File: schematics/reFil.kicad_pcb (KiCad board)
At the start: 2 copper layers, 19 parts, among them CON1 BARREL_JACK, P1 CONN_5X2, P2 CONN_2, P3 CONN_2, P4 CONN_2, U1 7805

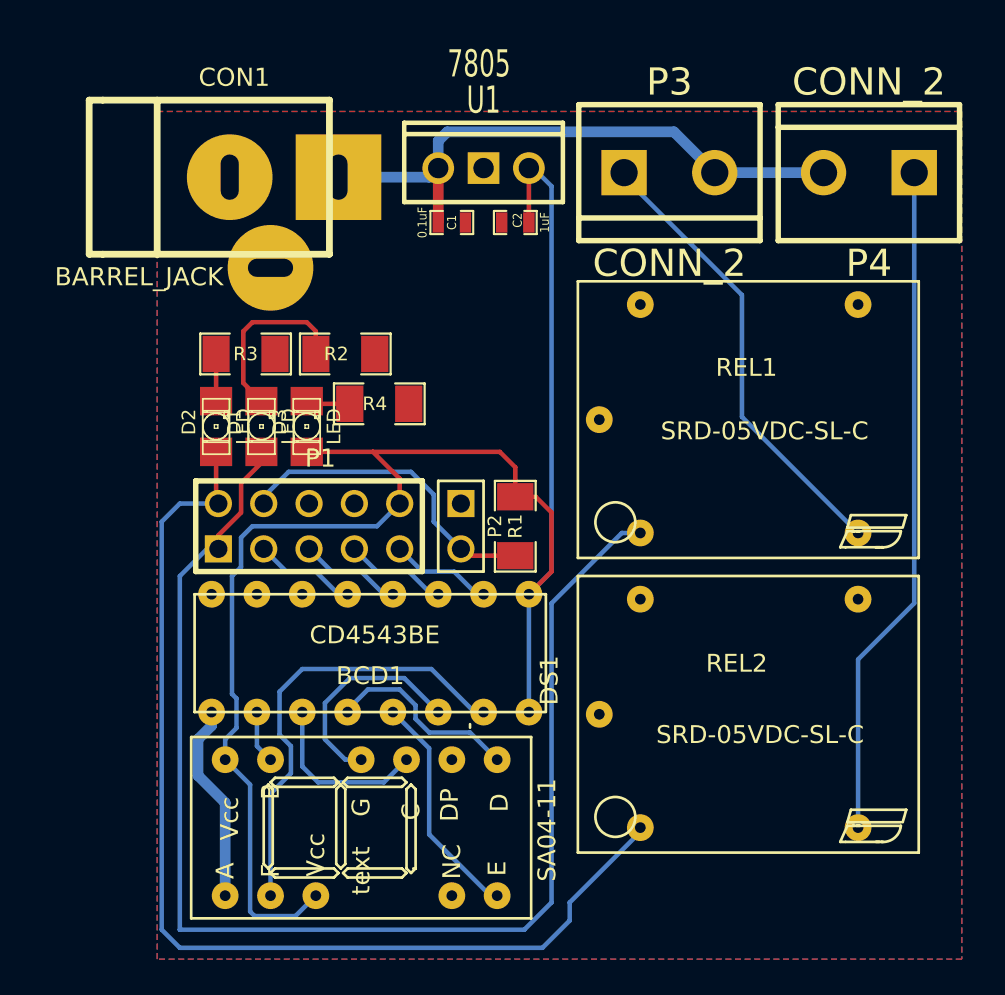
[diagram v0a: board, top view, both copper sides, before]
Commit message: Better layout
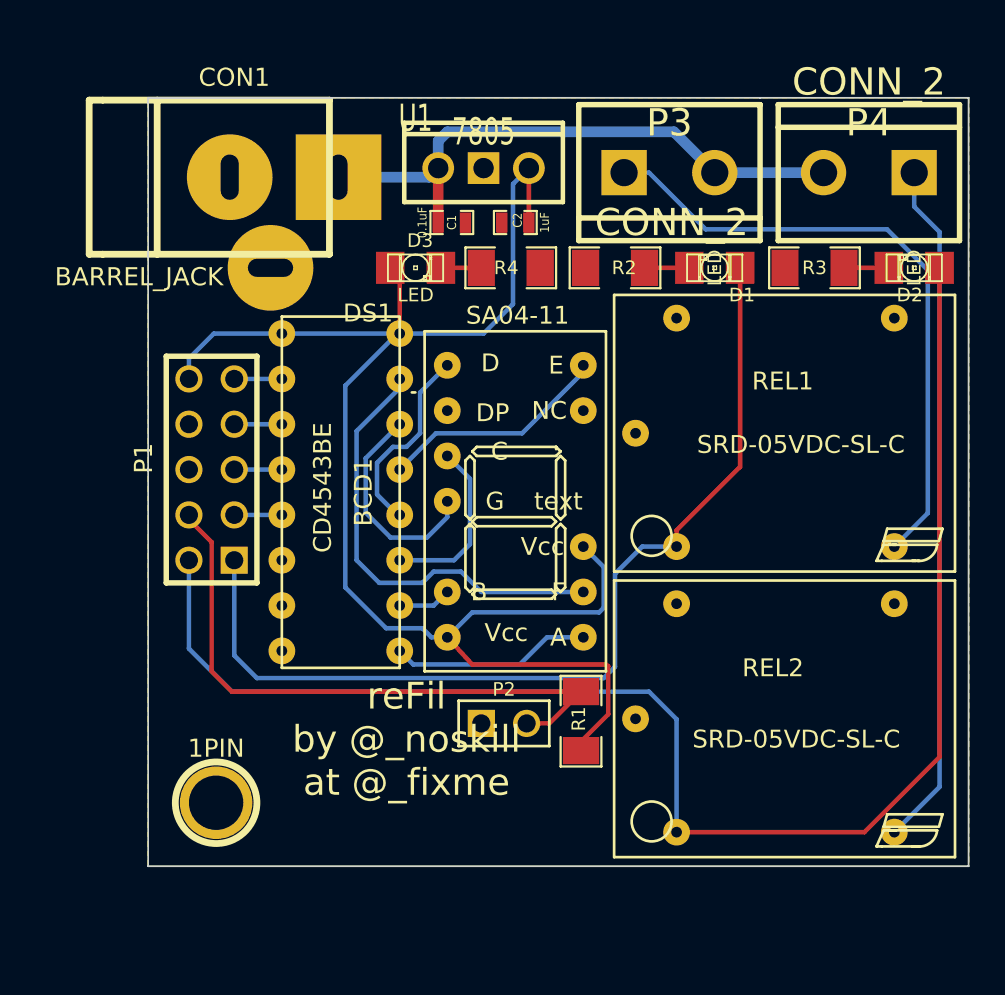
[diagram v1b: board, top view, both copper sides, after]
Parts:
- added 1PIN: P***, 1pin, F.Cu at (40.1, 66.0)
- moved D2 40.1 mm to (79.2, 36.1), turned to 180 degrees
- moved R3 32.2 mm to (73.7, 36.1), turned to 180 degrees
- moved D1 26.9 mm to (68.1, 36.1), turned to 180 degrees
- moved DS1 20.2 mm to (56.9, 49.1), turned to 180 degrees
- moved R2 15.9 mm to (62.5, 36.1), turned to 180 degrees
- moved R1 11.5 mm to (60.6, 61.5), turned to 90 degrees
- moved P2 11.3 mm to (56.3, 61.6), turned to 0 degrees
- moved D3 10.8 mm to (51.3, 36.1), turned to 0 degrees
- moved R4 10.6 mm to (56.6, 36.1)
- moved BCD1 9.17 mm to (47.1, 48.6), turned to 270 degrees
- moved P1 6.32 mm to (39.9, 47.4), turned to 90 degrees
- moved REL1 2.17 mm to (81.5, 53.1)
- moved REL2 2.05 mm to (81.5, 69.1)
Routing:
- net MOTOR: track 60.2 -> 84.1 mm
- net HEAT: track 73.9 -> 53.8 mm
- net TEMP: track 17.9 -> 34.2 mm
- net N-0000010: track 25.6 -> 35.5 mm
- net +5V: track 95.5 -> 86.4 mm
- net N-000006: track 10.1 -> 2.52 mm
- net C: track 5.75 -> 2.67 mm
- net B: track 5.75 -> 2.67 mm
- net D: track 5.75 -> 2.67 mm
- net A: track 5.75 -> 2.67 mm
- net N-000007: track 38.0 -> 38.6 mm
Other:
- board outline added: 46 x 43.1 mm
- board text added: "reFil by @_noskill at @_fixme"
